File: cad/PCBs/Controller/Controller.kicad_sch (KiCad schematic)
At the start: 20 parts, among them IC1 HT16K33, J3 Controller_Out, U3 BH1750FVI-TR, U4 HDC2080

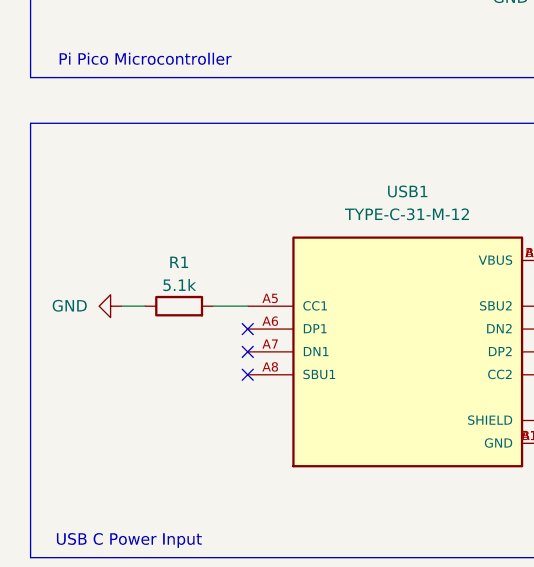
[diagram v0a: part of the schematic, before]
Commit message: WIP Routing Controller
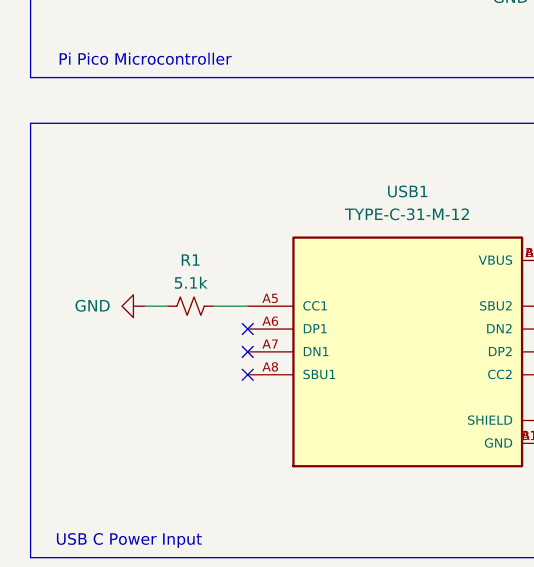
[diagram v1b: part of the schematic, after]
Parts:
- removed R1: 5.1k, Resistor_SMD:R_2010_5025Metric, symbol Device:R
- added R1: 5.1k, Resistor_SMD:R_0805_2012Metric, symbol Device:R_Small_US
- R2: footprint Resistor_SMD:R_2010_5025Metric -> Resistor_SMD:R_0805_2012Metric
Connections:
- net GND: now also R1.1
- net at USB1.A5 (CC1): now also R1.2
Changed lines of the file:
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@@
 	(wire
 		(pts
-			(xy 33.02 162.56) (xy 35.56 162.56)
+			(xy 35.56 162.56) (xy 38.1 162.56)
 		)
 		(stroke
@@
 	(label "MATRIX_SDA"
 		(at 204.47 120.65 180)
+		(fields_autoplaced yes)
 		(effects
 			(font
@@
 	(label "MATRIX_SCL"
 		(at 204.47 123.19 180)
+		(fields_autoplaced yes)
 		(effects
 			(font
@@
 	(label "MATRIX_SDA"
 		(at 99.06 72.39 0)
+		(fields_autoplaced yes)
 		(effects
 			(font
@@
 	(label "MATRIX_SCL"
 		(at 99.06 74.93 0)
+		(fields_autoplaced yes)
 		(effects
 			(font
@@
 	)
 	(symbol
-		(lib_id "Device:R")
-		(at 39.37 162.56 90)
-		(unit 1)
-		(exclude_from_sim no)
-		(in_bom yes)
-		(on_board yes)
-		(dnp no)
-		(property "Reference" "R1"
-			(at 39.37 157.734 90)
-			(effects
-				(font
-					(size 1.27 1.27)
-				)
-			)
-		)
-		(property "Value" "5.1k"
-			(at 39.37 160.274 90)
-			(effects
-				(font
-					(size 1.27 1.27)
-				)
-			)
-		)
-		(property "Footprint" "Resistor_SMD:R_2010_5025Metric"
-			(at 39.37 164.338 90)
-			(effects
-				(font
-					(size 1.27 1.27)
-				)
-				(hide yes)
-			)
-		)
-		(property "Datasheet" "~"
-			(at 39.37 162.56 0)
-			(effects
-				(font
-					(size 1.27 1.27)
-				)
-				(hide yes)
-			)
-		)
-		(property "Description" "Resistor"
-			(at 39.37 162.56 0)
-			(effects
-				(font
-					(size 1.27 1.27)
-				)
-				(hide yes)
-			)
-		)
-		(pin "1"
-		)
-		(pin "2"
-		)
-		(instances
-			(project "RGB_Segment_Clock"
-				(path "/40bfd19c-28ae-4125-bffd-c1ba01268b82/ddbd17b6-28a0-495f-a062-2182329bea65"
-					(reference "R1")
-					(unit 1)
-				)
-			)
-		)
-	)
-	(symbol
 		(lib_id "Device:R_Small_US")
 		(at 214.63 41.91 180)
@@
 			)
 		)
-		(property "Footprint" "Resistor_SMD:R_2010_5025Metric"
+		(property "Footprint" "Resistor_SMD:R_0805_2012Metric"
 			(at 88.9 170.18 0)
 			(effects
@@
 	(symbol
 		(lib_id "power:GND")
-		(at 33.02 162.56 270)
+		(at 35.56 162.56 270)
 		(unit 1)
 		(exclude_from_sim no)
@@
 		(fields_autoplaced yes)
 		(property "Reference" "#PWR01"
-			(at 26.67 162.56 0)
+			(at 29.21 162.56 0)
 			(effects
 				(font
@@
 		)
 		(property "Value" "GND"
-			(at 29.21 162.5599 90)
+			(at 31.75 162.5599 90)
 			(effects
 				(font
@@
 		)
 		(property "Footprint" ""
-			(at 33.02 162.56 0)
+			(at 35.56 162.56 0)
 			(effects
 				(font
@@
 		)
 		(property "Datasheet" ""
-			(at 33.02 162.56 0)
+			(at 35.56 162.56 0)
 			(effects
 				(font
@@
 		)
 		(property "Description" "Power symbol creates a global label with name \"GND\" , ground"
-			(at 33.02 162.56 0)
+			(at 35.56 162.56 0)
 			(effects
 				(font
@@
 					(unit 1)
 				)
+			)
+		)
+	)
+	(symbol
+		(lib_id "Device:R_Small_US")
+		(at 40.64 162.56 90)
+		(unit 1)
+		(exclude_from_sim no)
+		(in_bom yes)
+		(on_board yes)
+		(dnp no)
+		(property "Reference" "R1"
+			(at 40.64 157.48 90)
+			(effects
+				(font
+					(size 1.27 1.27)
+				)
+			)
+		)
+		(property "Value" "5.1k"
+			(at 40.64 160.02 90)
+			(effects
+				(font
+					(size 1.27 1.27)
+				)
+			)
+		)
+		(property "Footprint" "Resistor_SMD:R_0805_2012Metric"
+			(at 40.64 162.56 0)
+			(effects
+				(font
+					(size 1.27 1.27)
+				)
+				(hide yes)
+			)
+		)
+		(property "Datasheet" "~"
+			(at 40.64 162.56 0)
+			(effects
+				(font
+					(size 1.27 1.27)
+				)
+				(hide yes)
+			)
+		)
+		(property "Description" "Resistor, small US symbol"
+			(at 40.64 162.56 0)
+			(effects
+				(font
+					(size 1.27 1.27)
+				)
+				(hide yes)
+			)
+		)
+		(pin "1"
+		)
+		(pin "2"
+		)
+		(instances
+			(project "RGB_Segment_Clock"
+				(path "/40bfd19c-28ae-4125-bffd-c1ba01268b82/ddbd17b6-28a0-495f-a062-2182329bea65"
+					(reference "R1")
+					(unit 1)
+				)

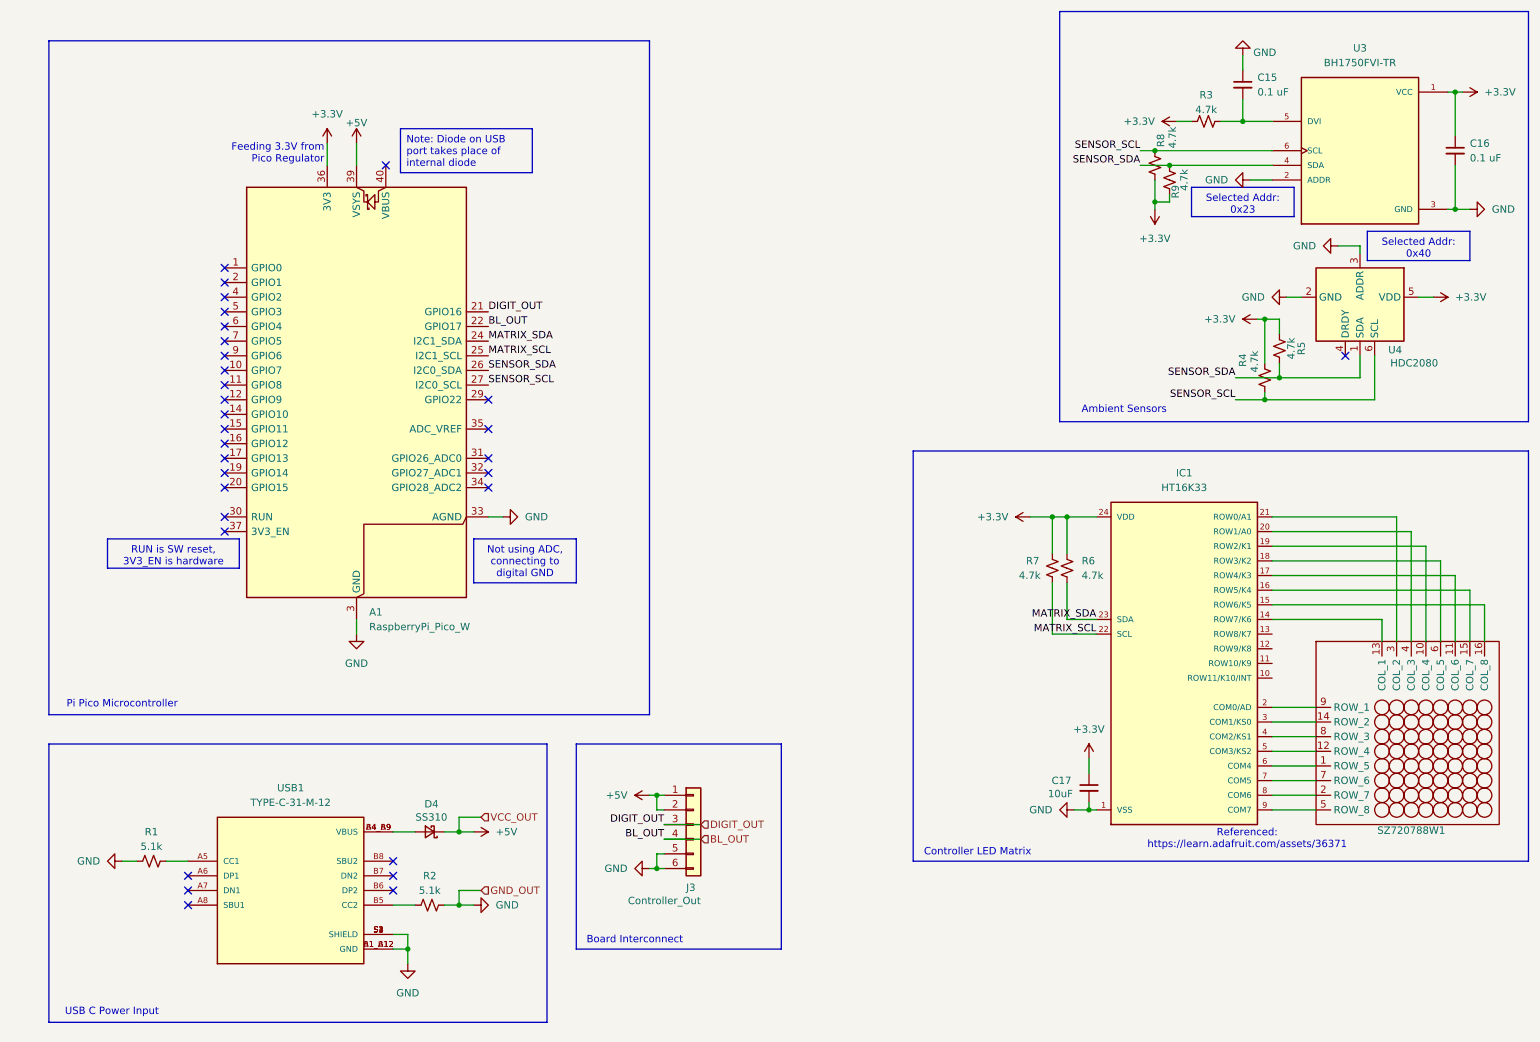
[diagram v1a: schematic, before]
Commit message: WIP Integrating USB C PD
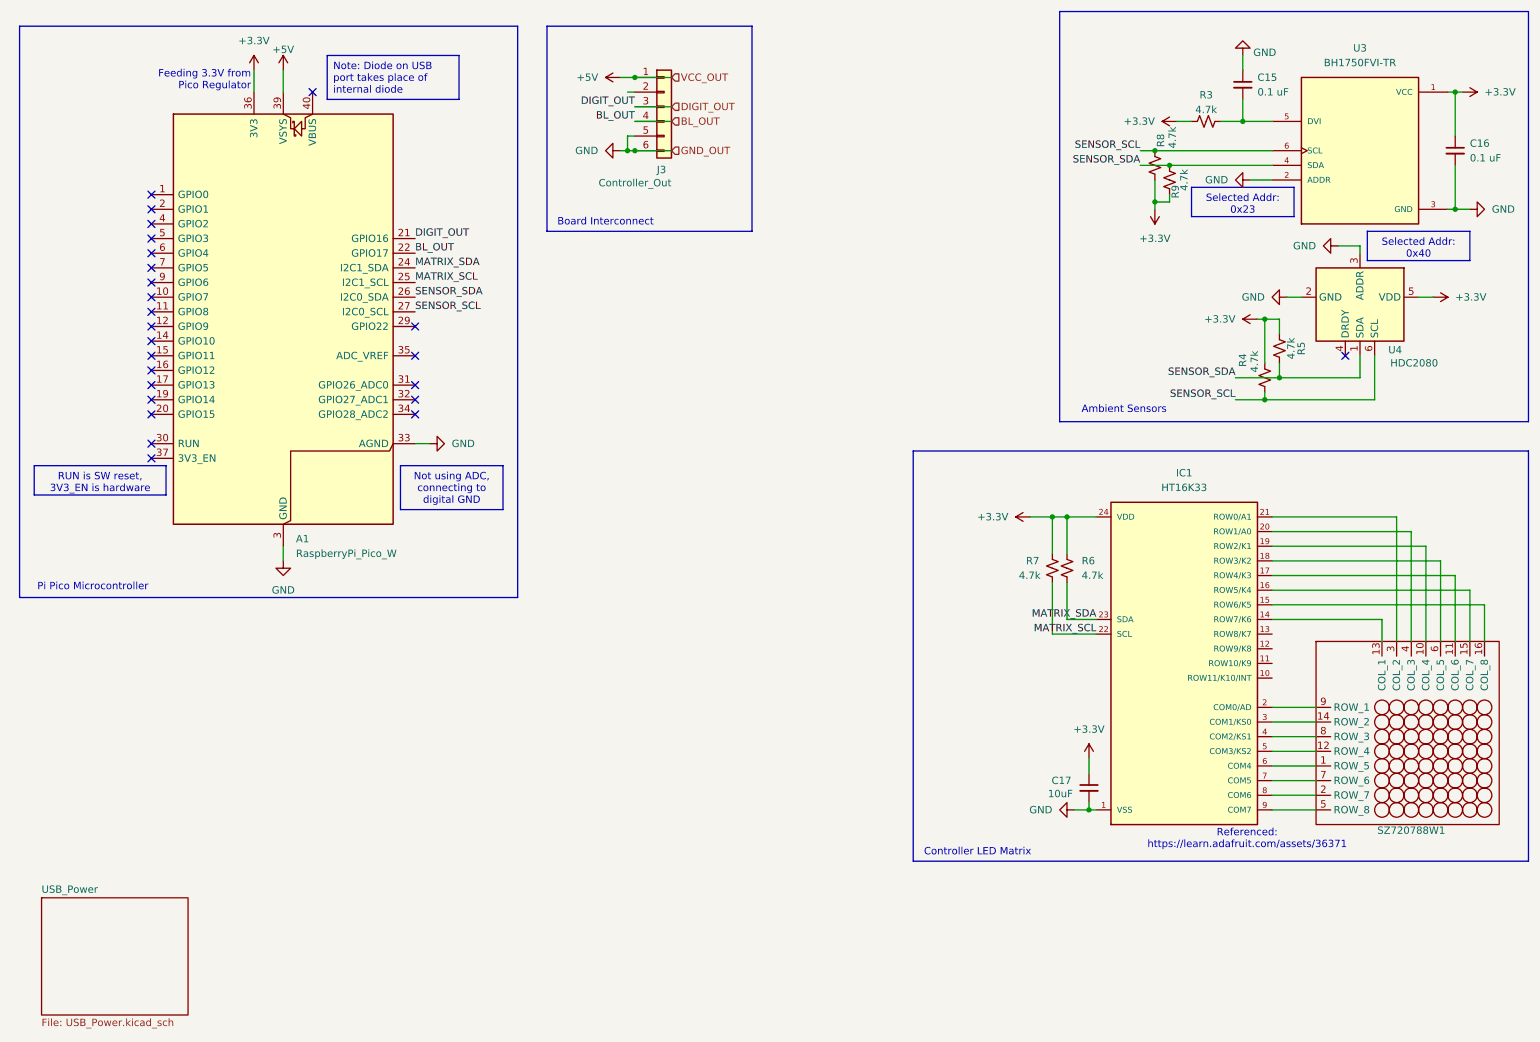
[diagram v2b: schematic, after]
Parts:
- removed D4: SS310, Diode_SMD:D_SOD-323F, symbol Device:D_Schottky_Small
- removed R1, R2: 5.1k, Resistor_SMD:R_0805_2012Metric, symbol Device:R_Small_US
- removed USB1: TYPE-C-31-M-12, TYPE-C-31-M-12:HRO_TYPE-C-31-M-12, symbol TYPE-C-31-M-12:TYPE-C-31-M-12
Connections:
- net +5V: no longer J3.2 (Pin_2)
- no-connect marks 31 -> 25
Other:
- added sheet USB_Power (USB_Power.kicad_sch)
- note removed: "USB C Power Input"
- moved on the sheet: A1, J3
